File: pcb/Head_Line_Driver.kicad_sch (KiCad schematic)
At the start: 9 parts

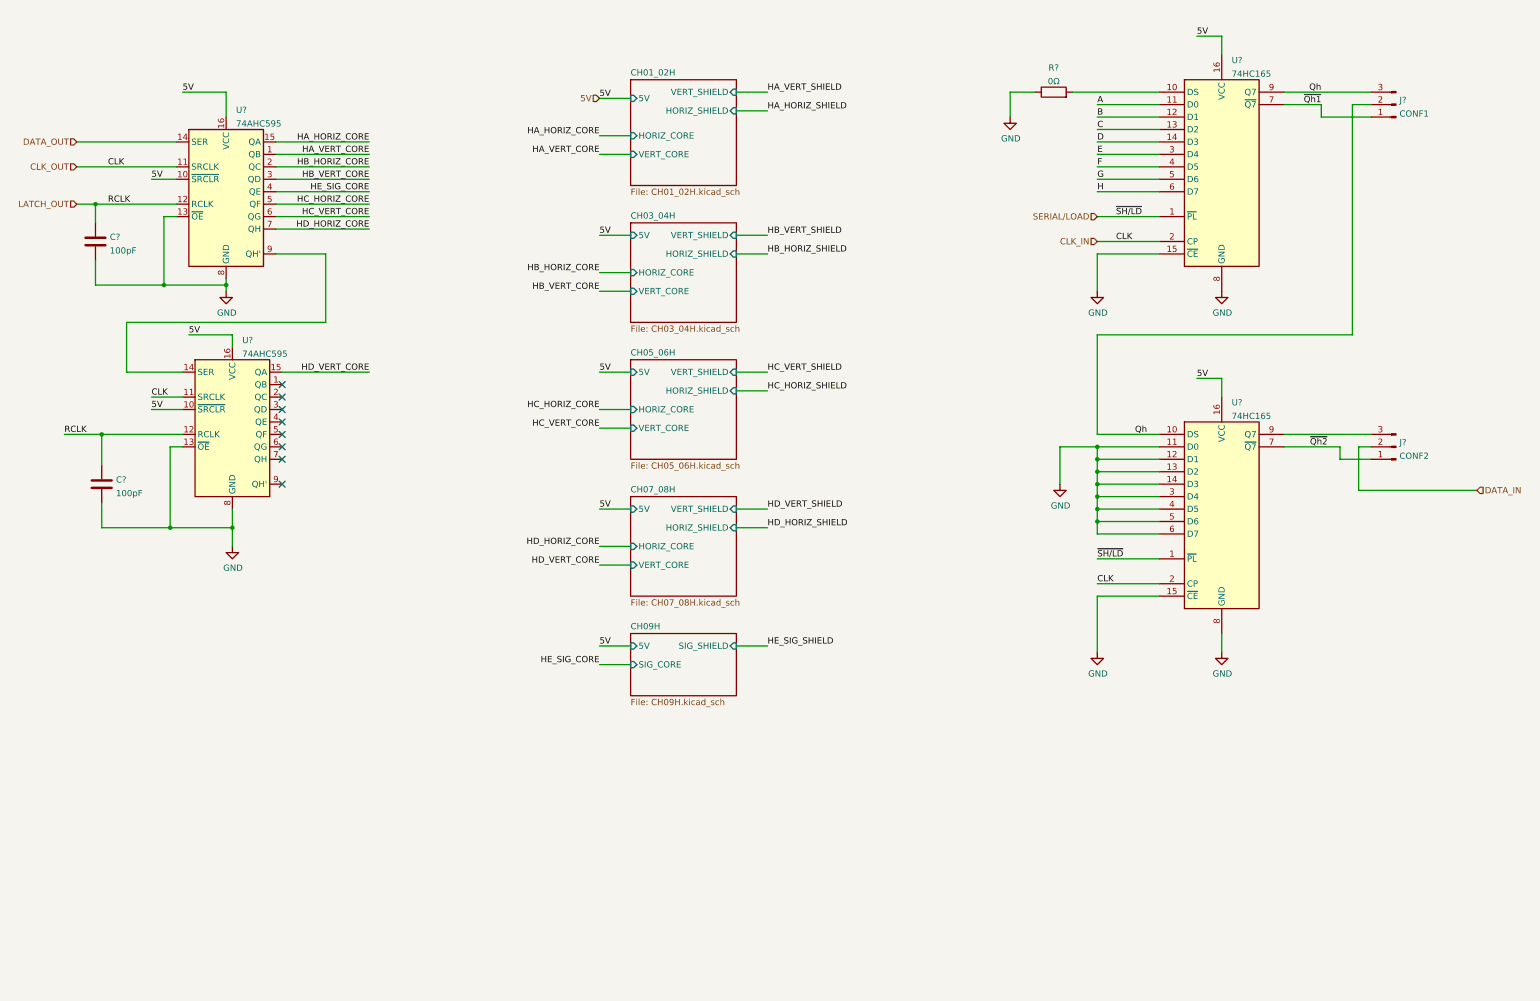
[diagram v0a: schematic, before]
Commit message: Updates to the shematic for mechanics
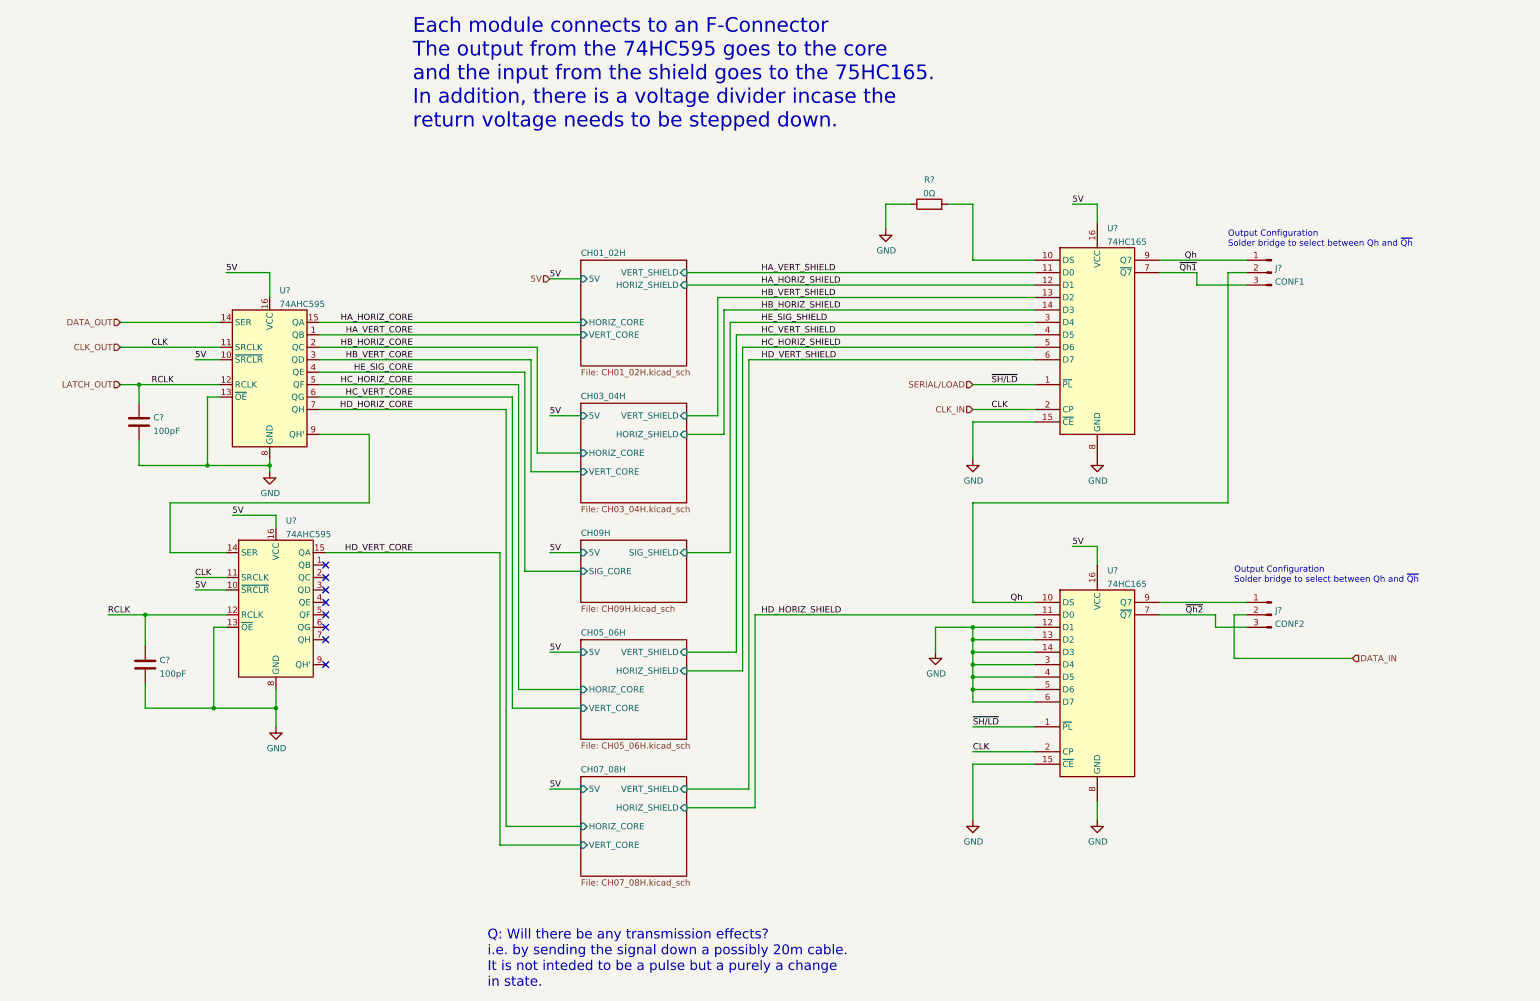
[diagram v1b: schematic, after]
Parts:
- C? (x2): footprint (none) -> Capacitor_SMD:C_0805_2012Metric
- J? (x2): footprint (none) -> Jumper:SolderJumper-3_P1.3mm_Bridged12_RoundedPad1.0x1.5mm
- R?: footprint (none) -> Resistor_SMD:R_0805_2012Metric
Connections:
- net A is gone; now on net HA_VERT_SHIELD: U?.11 (D0)
- net B is gone; now on net HA_HORIZ_SHIELD: U?.12 (D1)
- net C is gone; now on net HB_VERT_SHIELD: U?.13 (D2)
- net D is gone; now on net HB_HORIZ_SHIELD: U?.14 (D3)
- net E is gone; now on net HE_SIG_SHIELD: U?.3 (D4)
- net F is gone; now on net HC_VERT_SHIELD: U?.4 (D5)
- net G is gone; now on net HC_HORIZ_SHIELD: U?.5 (D6)
- net H is gone; now on net HD_VERT_SHIELD: U?.6 (D7)
- net GND: no longer U?.11 (D0)
- net HD_HORIZ_SHIELD: now also U?.11 (D0)
- net Qh: now also J?.1 (Pin_1); no longer J?.3 (Pin_3)
- net ~{Qh1}: now also J?.3 (Pin_3); no longer J?.1 (Pin_1)
- net ~{Qh2}: now also J?.3 (Pin_3); no longer J?.1 (Pin_1)
- net at U?.9 (Q7): now also J?.1 (Pin_1); no longer J?.3 (Pin_3)
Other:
- note added: "Each module connects to an F-Connector The output from the 74HC595 goes to the core and the input from the shield goes to the 75HC165. In addition, there is a voltage divider incase the return voltage needs to be stepped down."
- note added: "Output Configuration Solder bridge to select between Qh and ~{Qh}"
- note added: "Q: Will there be any transmission effects? i.e. by sending the signal down a possibly 20m cable. It is not inteded to be a pulse but a purely a change in state."
- moved on the sheet: C?, J?, R?, U?
